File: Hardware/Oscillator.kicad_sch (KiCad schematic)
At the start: 0 parts

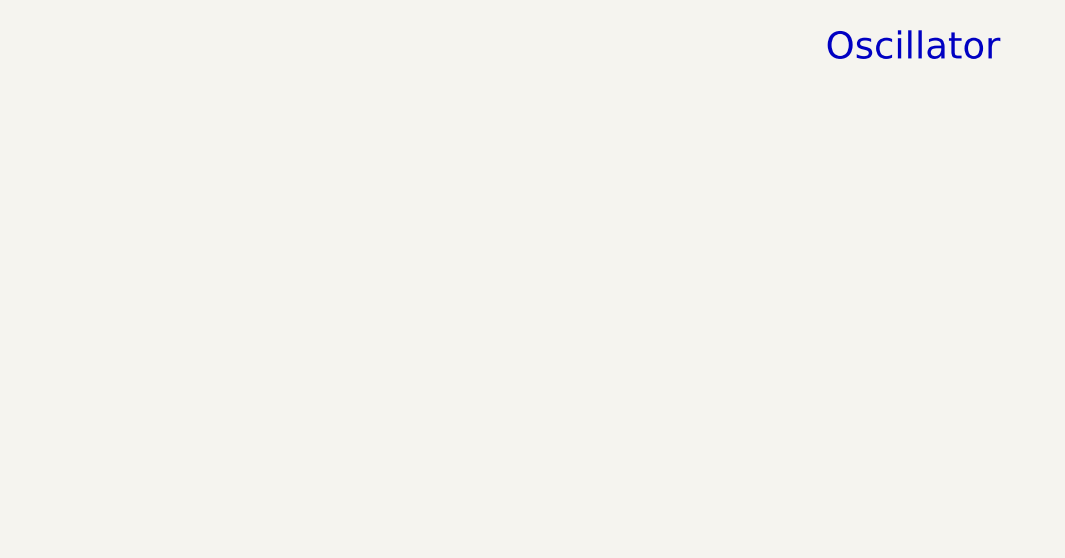
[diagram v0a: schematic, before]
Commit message: More WIP
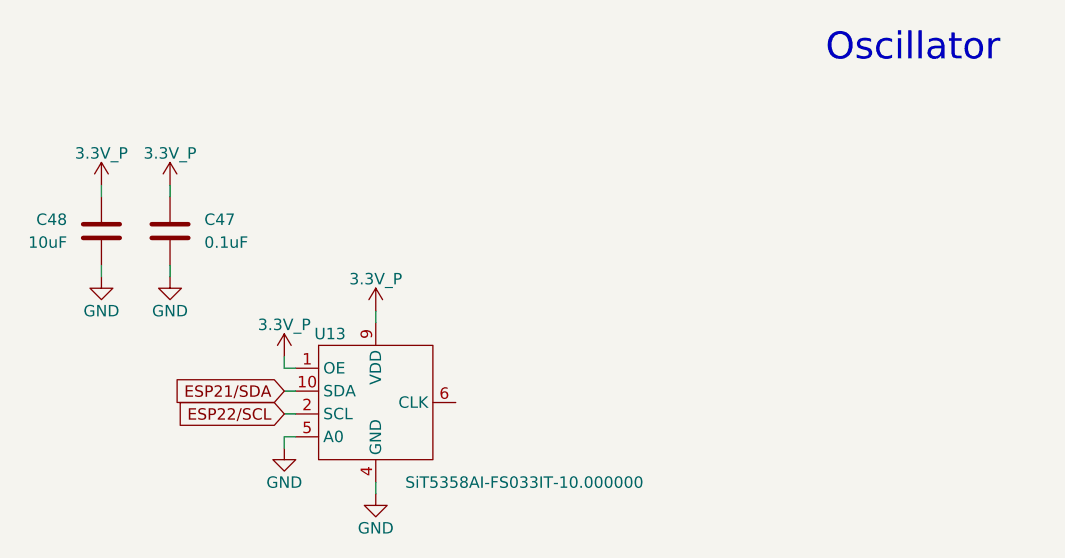
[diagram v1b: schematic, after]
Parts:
- added C47: 0.1uF, SparkFun-Capacitor:C_0603_1608Metric, symbol SparkFun-Capacitor:0.1uF_0603_25V_20%
- added C48: 10uF, SparkFun-Capacitor:C_0603_1608Metric, symbol SparkFun-Capacitor:10uF_0603_10V_20%
- added U13: SiT5358AI-FS033IT-10.000000, SparkFun-Semiconductor-Standard:Ceramic_QFN_5.0x3.2mm-10, symbol SparkFun-Clock:SiT5358_TCXO_10MHz_5.0x3.2mm
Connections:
- new net 3.3V_P: C47.1, C48.1, U13.1 (OE), U13.9 (VDD)
- new net ESP21/SDA: U13.10 (SDA)
- new net ESP22/SCL: U13.2 (SCL)
- new net GND: C47.2, C48.2, U13.4 (GND), U13.5 (A0)

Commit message: More WIP
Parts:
- removed C47: 0.1uF, SparkFun-Capacitor:C_0603_1608Metric, symbol SparkFun-Capacitor:0.1uF_0603_25V_20%
- removed C48: 10uF, SparkFun-Capacitor:C_0603_1608Metric, symbol SparkFun-Capacitor:10uF_0603_10V_20%
- removed U13: SiT5358AI-FS033IT-10.000000, SparkFun-Semiconductor-Standard:Ceramic_QFN_5.0x3.2mm-10, symbol SparkFun-Clock:SiT5358_TCXO_10MHz_5.0x3.2mm
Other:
- note removed: "Oscillator"
